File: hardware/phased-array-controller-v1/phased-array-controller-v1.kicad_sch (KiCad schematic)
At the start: 9 parts, among them IC1 WP4U+, IC2 WP4U+, IC3 WP4U+, IC4 WP4U+, IC5 WP4U+, J1 Conn_Coaxial, U1 SKY13330-397LF

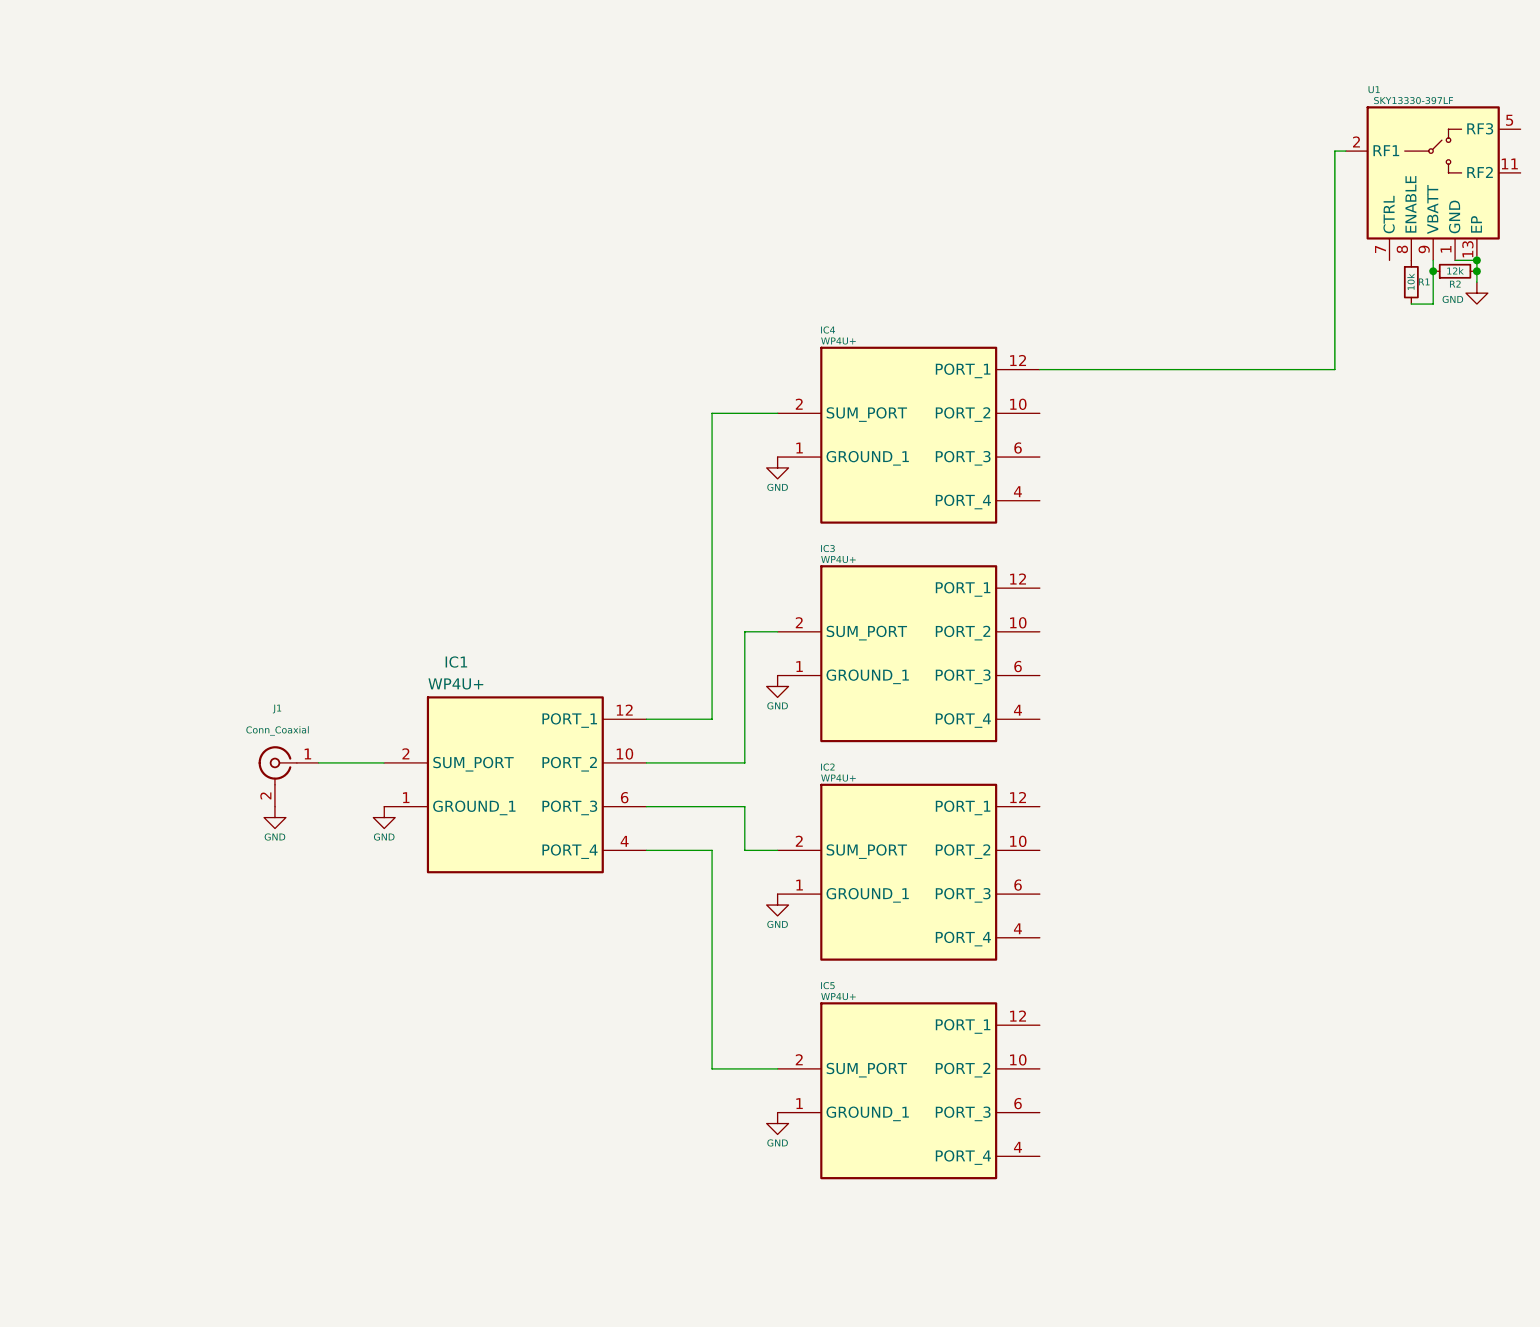
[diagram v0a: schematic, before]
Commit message: updates
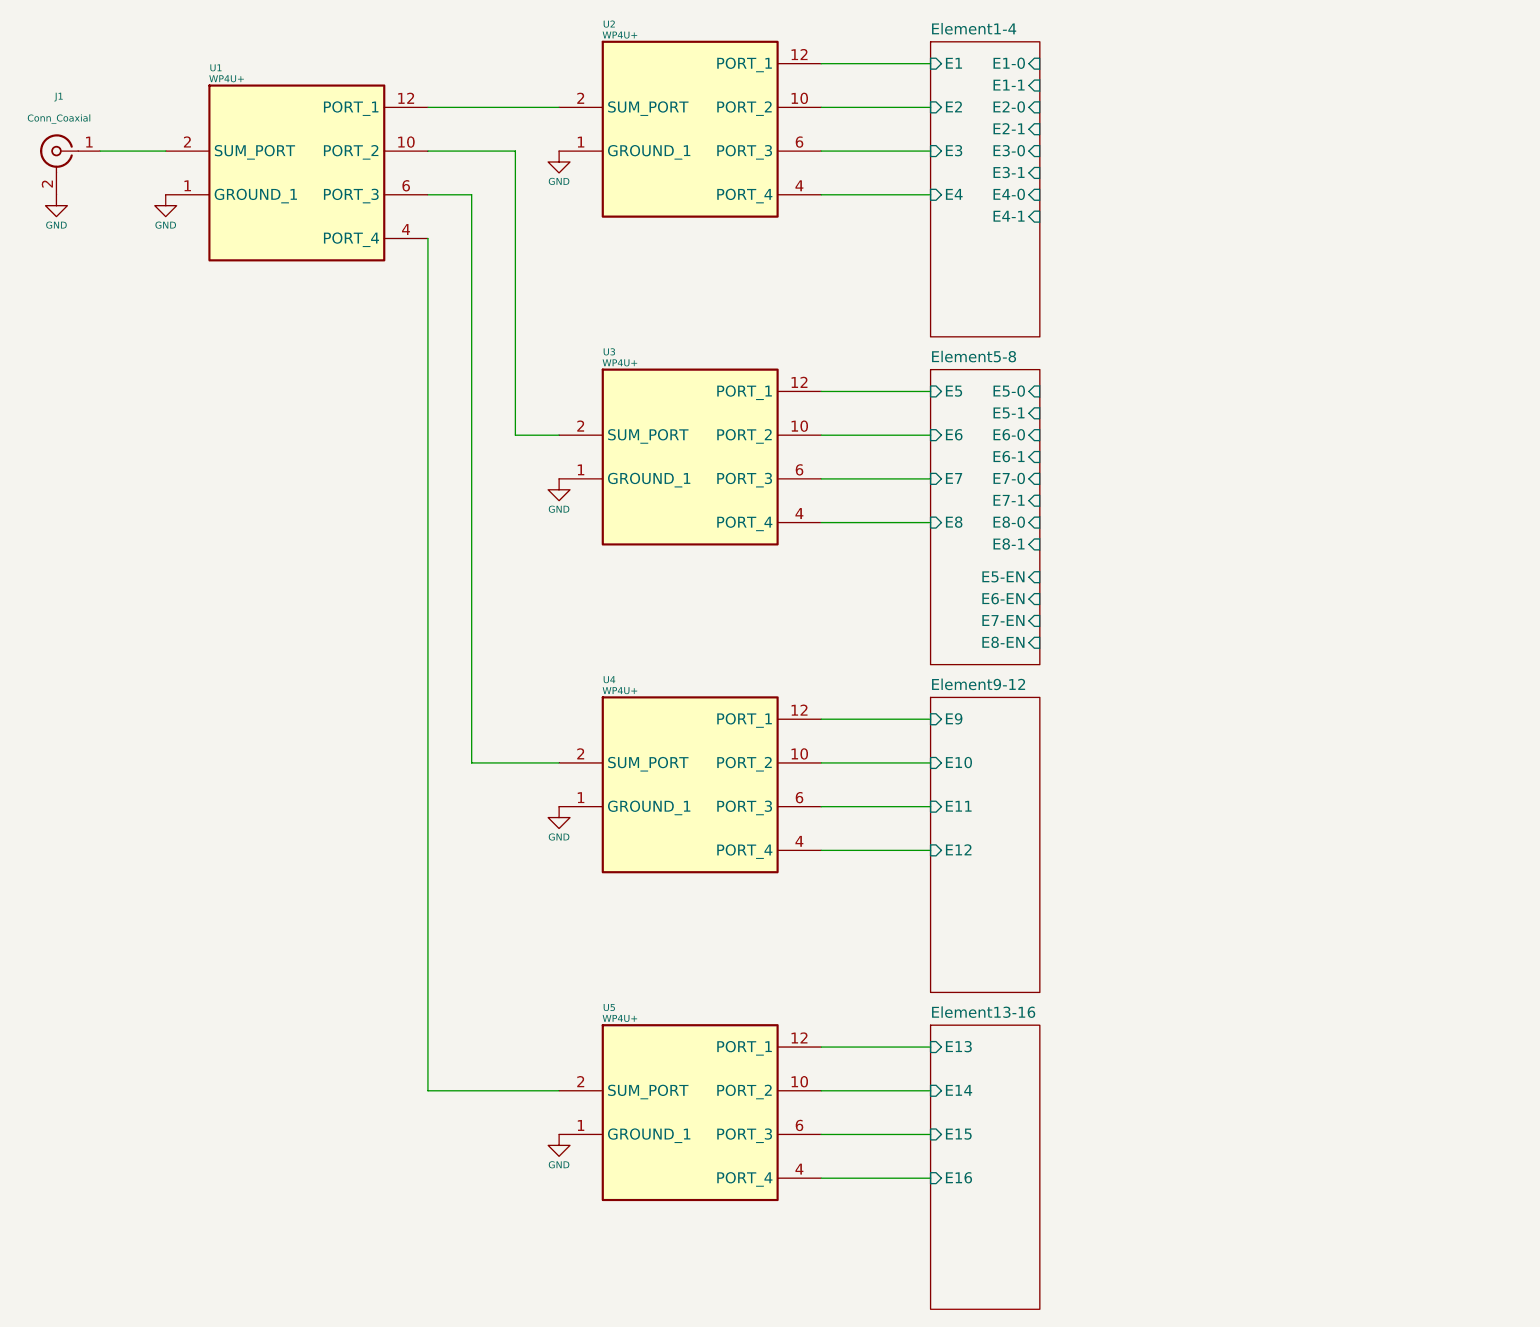
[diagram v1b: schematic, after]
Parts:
- removed IC1: WP4U+, QFN51P300X300X89-13N, symbol phased-array:WP4U+
- removed R1: 10k, Resistor_SMD:R_0603_1608Metric, symbol Device:R_Small
- removed R2: 12k, Resistor_SMD:R_0603_1608Metric, symbol Device:R_Small
- removed U1: SKY13330-397LF, SKY13330397LF, symbol phased-array:SKY13330-397LF
- added U1: WP4U+, QFN51P300X300X89-13N, symbol phased-array:WP4U+
- renumbered IC4 to U2, IC3 to U3, IC2 to U4, IC5 to U5
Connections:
- net GND: now also U1.1 (GROUND_1), U1.11 (GROUND_7), U1.13 (GROUND_8), U1.3 (GROUND_2), U1.5 (GROUND_3), U1.7 (GROUND_4), U1.8 (GROUND_5), U1.9 (GROUND_6)
- net Element9-12/E10: now reaches U4.10 (PORT_2)
- net Element9-12/E9: now reaches U4.12 (PORT_1)
- net at U4.2 (SUM_PORT): now also U1.6 (PORT_3)
- net Element9-12/E12: now reaches U4.4 (PORT_4)
- net Element9-12/E11: now reaches U4.6 (PORT_3)
- net Element1-4/E1: now reaches U2.12 (PORT_1)
- net Element1-4/E2: now reaches U2.10 (PORT_2)
- net at U2.2 (SUM_PORT): now also U1.12 (PORT_1)
- net Element1-4/E4: now reaches U2.4 (PORT_4)
- net Element1-4/E3: now reaches U2.6 (PORT_3)
- net Element5-8/E6: now reaches U3.10 (PORT_2)
- net Element5-8/E5: now reaches U3.12 (PORT_1)
- net at U3.2 (SUM_PORT): now also U1.10 (PORT_2)
- net Element5-8/E8: now reaches U3.4 (PORT_4)
- net Element5-8/E7: now reaches U3.6 (PORT_3)
- net Element13-16/E14: now reaches U5.10 (PORT_2)
- net Element13-16/E13: now reaches U5.12 (PORT_1)
- net at U5.2 (SUM_PORT): now also U1.4 (PORT_4)
- net Element13-16/E16: now reaches U5.4 (PORT_4)
- net Element13-16/E15: now reaches U5.6 (PORT_3)
- net at J1.1 (In): now also U1.2 (SUM_PORT)
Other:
- added sheet Element1-4 (E1-4.kicad_sch)
- added sheet Element13-16 (E13-16.kicad_sch)
- added sheet Element5-8 (E5-8.kicad_sch)
- added sheet Element9-12 (E9-12.kicad_sch)
- moved on the sheet: J1, U2, U3, U4, U5
